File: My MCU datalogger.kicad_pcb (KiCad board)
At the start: 2 copper layers, 47.7 x 30.6 mm, 29 parts, among them J1 Conn_01x04_Male, J2 Conn_01x09_Male, J3 Conn_01x04_Male, J4 Conn_02x03_Odd_Even, U1 24LC1025, U2 DS1307Z, U3 24LC1025, U4 ATMEGA328P-AU, Y1 32.768 KHz, Y2 16 MHz

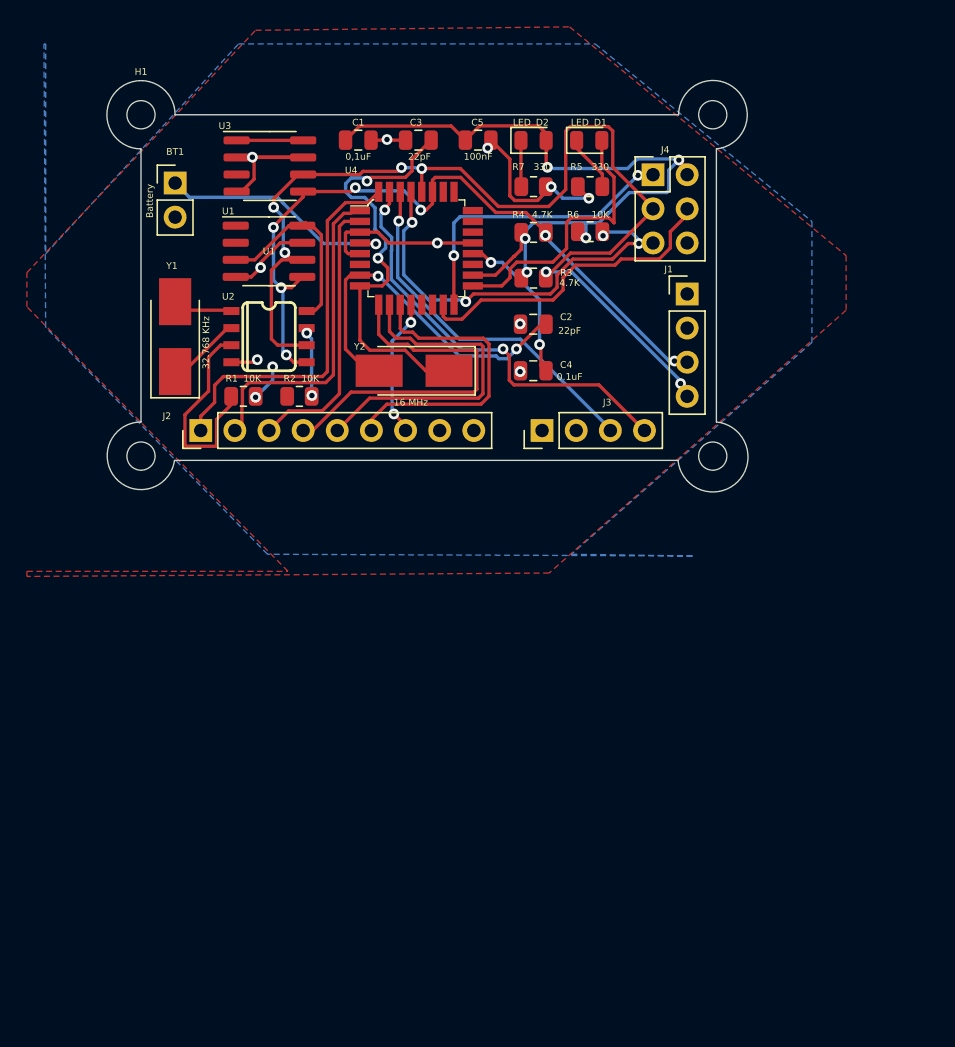
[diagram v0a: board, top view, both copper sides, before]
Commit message: Generated Gerbers files
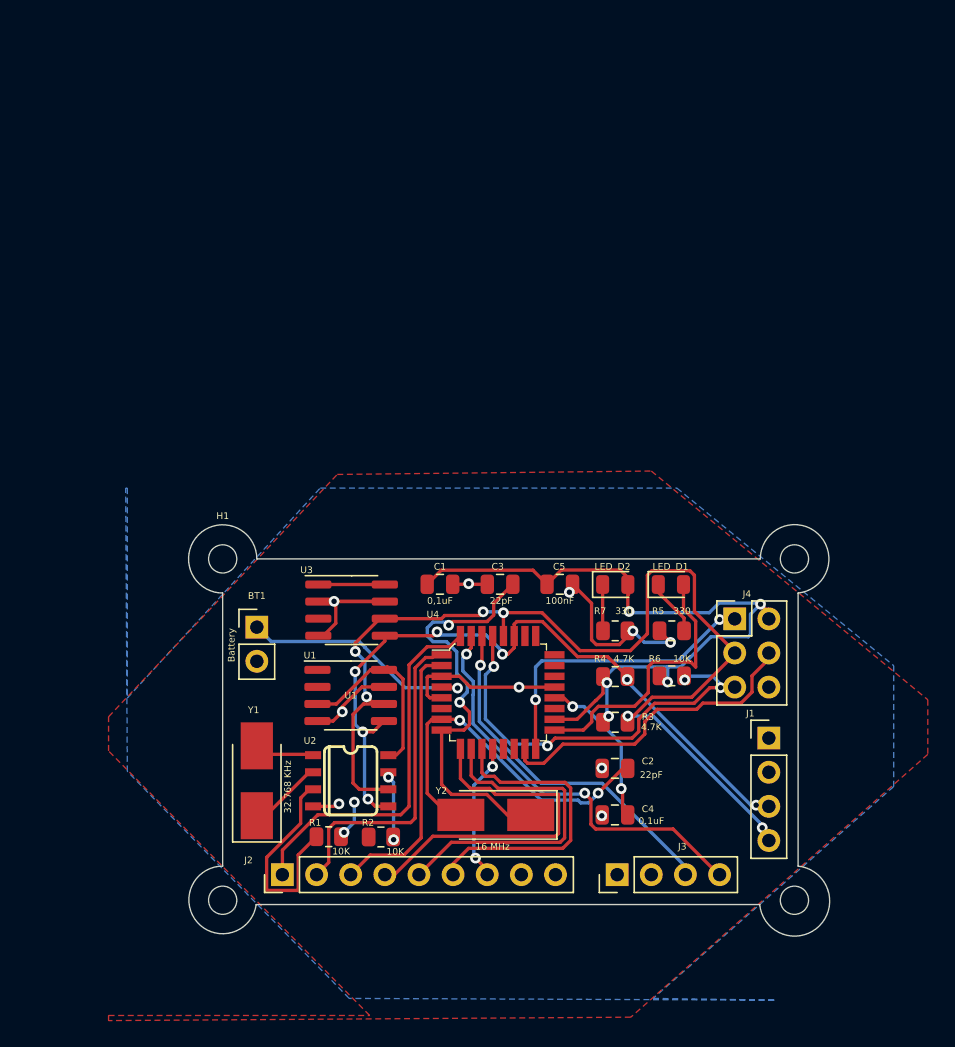
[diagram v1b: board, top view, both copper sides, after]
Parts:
- added G***: LOGO, 4x8x8 matrix display:TE_Logo_11.6x4, B.Cu at (64.5, 75.2)
- added REF**: KiCad-Logo2_5mm_SilkScreen, Symbol:KiCad-Logo2_5mm_SilkScreen, B.Cu at (55.9, 60.7)
- moved C2 33.6 mm to (74.2, 73.0)
- moved H2 33.6 mm to (45.1, 82.8)
- moved H4 33.6 mm to (87.6, 82.8)
- moved J1 33.6 mm to (85.7, 70.7)
- moved R3 33.6 mm to (74.3, 69.5)
- moved R4 33.6 mm to (74.3, 66.1)
- moved U2 33.6 mm to (54.6, 73.9)
- moved Y1 33.6 mm to (47.6, 73.9)
- moved BT1 33.6 mm to (47.6, 62.4)
- moved C1 33.6 mm to (61.2, 59.3)
- moved C3 33.6 mm to (65.7, 59.3)
- moved C5 33.6 mm to (70.1, 59.3)
- moved D1 33.6 mm to (78.4, 59.3)
- moved D2 33.6 mm to (74.3, 59.3)
- moved H1 33.6 mm to (45.1, 57.4)
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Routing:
- net Net-(R1-Pad2): track 15.3 -> 16.0 mm
- net /D2: track 28.5 -> 27.8 mm
- net /TX: track 31.8 -> 31.2 mm
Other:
- board text added: "0.2000 mm / 0.0000 mm"
- board text added: "0.3000 mm"
- board text added: "1.6000 mm"
- board text added: "2"
- board text added: "47.7044 mm x 30.6182 mm"
- board text added: "BOARD CHARACTERISTICS"
- board text added: "Board Thickness:"
- board text added: "Board overall dimensions:"
- board text added: "Castellated pads:"
- board text added: "Copper Finish:"
- board text added: "Copper Layer Count:"
- board text added: "Data logger with the ATMega328P. - 2Mbit EEPROM - RTC - I2C, SPI, GPIOs"
- board text added: "Edge card connectors:"
- board text added: "Impedance Control:"
- board text added: "Min hole diameter:"
- board text added: "Min track/spacing:"
- board text added: "No"
- board text added: "None"
- board text added: "PCB V. ${design_version}"
- board text added: "Plated Board Edge:"

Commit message: 4_layers final candidate
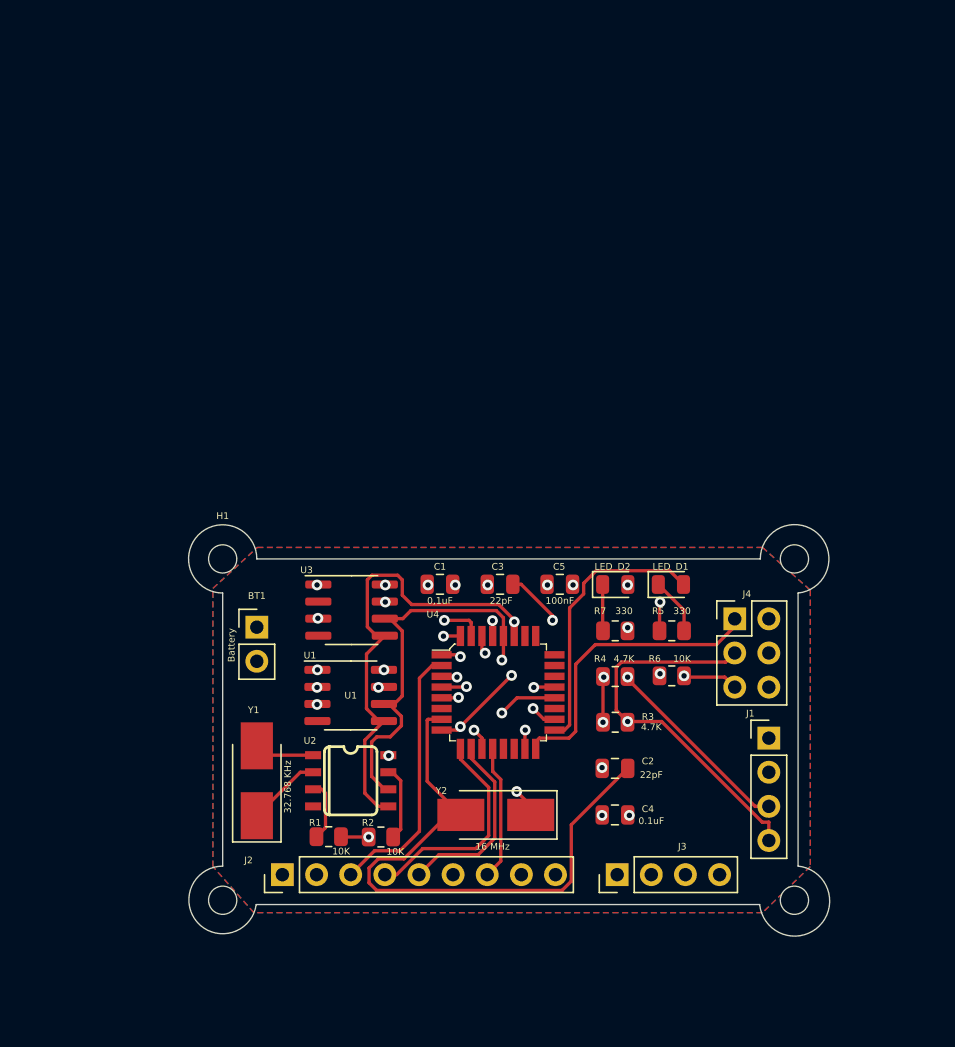
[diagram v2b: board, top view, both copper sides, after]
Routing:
- net /Vcc: track 96.3 -> 9.59 mm, vias 8 -> 17
- net GND: track 48.0 -> 7.26 mm, vias 10 -> 12
- net Net-(C2-Pad2): track 27.0 -> 44.4 mm, vias 2 -> 0
- net Net-(R1-Pad2): track 16.0 -> 4.56 mm
- net /SCK: track 83.1 -> 71.8 mm, vias 6 -> 2
- net /D5: track 27.1 -> 16.3 mm
- net /D6: track 24.9 -> 14.1 mm
- net /RESET: track 30.7 -> 22.7 mm, vias 4 -> 2
- net /D7: track 23.0 -> 15.5 mm, vias 0 -> 1
- net Net-(C4-Pad2): track 11.2 -> 18.3 mm
- net Net-(C3-Pad2): track 31.8 -> 25.3 mm, vias 2 -> 4
- net /SDA: track 54.6 -> 60.8 mm, vias 7 -> 2
- net /TX: track 31.2 -> 37.3 mm, vias 2 -> 1
- net /D2: track 27.8 -> 24.0 mm, vias 0 -> 1
- net /MOSI: track 24.0 -> 22.4 mm, vias 0 -> 1
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- added copper zone on In1.Cu, net /Vcc
- added copper zone on F.Cu, net GND
- removed copper zone on F.Cu, net /Vcc
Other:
- copper layers 2 -> 4
